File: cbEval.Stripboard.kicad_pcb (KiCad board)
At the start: 2 copper layers, 35 x 109 mm, 33 parts, among them J1 Bergstik-II_3, J10 Socket.Hor.2x5.6-5535512-4, J11 Bergstik-II_3, J12 Bergstik-II_3, J13 Bergstik-II_6, J14 Bergstik-II_8, J15 Bergstik-II_6, J2 Bergstik-II_6, J3 Keystone.4918, J4 Keystone.4918, J5 Keystone.3571, J6 Keystone.3571, J7 Socket.Hor.2x5.6-5535512-4, J8 Header.Hor.2x5.9-103326-0-05, J9 Header.Hor.2x5.9-103326-0-05, U1 SN74AHC138D

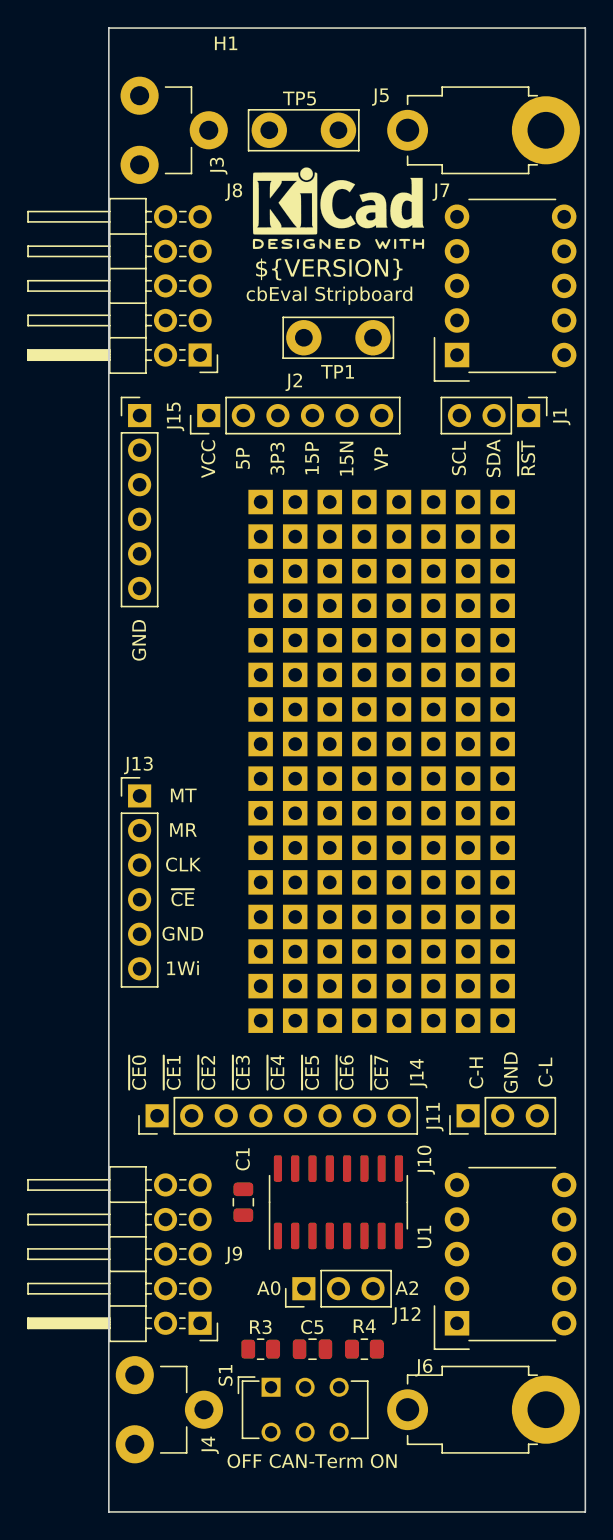
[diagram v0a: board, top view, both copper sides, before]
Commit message: Bus-Stecker getauscht, BOM erstellt
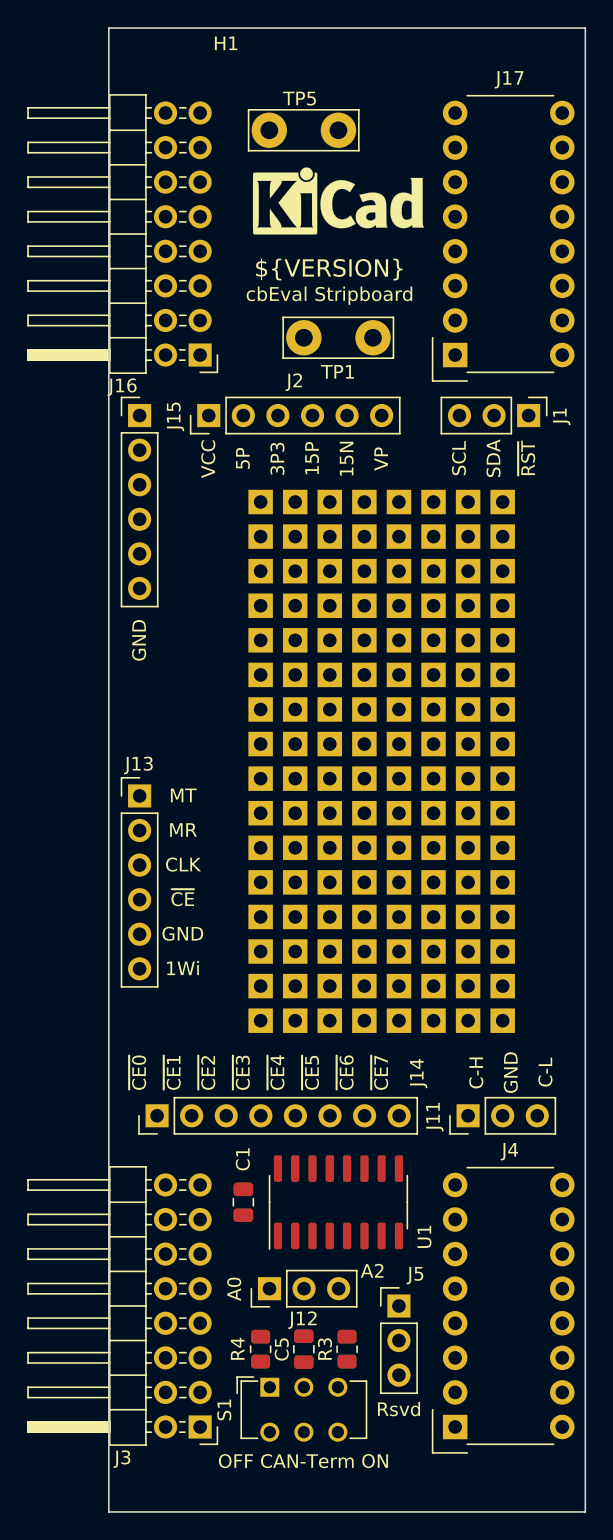
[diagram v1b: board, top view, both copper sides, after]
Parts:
- removed J10, J7: Socket.Hor.2x5.6-5535512-4, BTech.Connector.AMPMODU-ModII:Socket.Hor.2x5.6-5535512-4
- removed J6: Keystone.3571, BTech.Connector.QuickConnect:Keystone.3571
- removed J8, J9: Header.Hor.2x5.9-103326-0-05, Connector_PinHeader_2.54mm:PinHeader_2x05_P2.54mm_Horizontal
- added J16: Header.Hor.2x8.9-103326-0-08, Connector_PinHeader_2.54mm:PinHeader_2x08_P2.54mm_Horizontal, F.Cu at (135.3, 70.5)
- added J17: Socket.Hor.2x8.1-5535512-8, BTech.Connector.AMPMODU-ModII:Socket.Hor.2x5.6-5535512-4, F.Cu at (161.9, 62.9)
- J3: value Keystone.4918 -> Header.Hor.2x8.9-103326-0-08; footprint BTech.Connector.QuickConnect:Keystone.4918 -> Connector_PinHeader_2.54mm:PinHeader_2x08_P2.54mm_Horizontal
- J4: value Keystone.4918 -> Socket.Hor.2x8.1-5535512-8; footprint BTech.Connector.QuickConnect:Keystone.4918 -> BTech.Connector.AMPMODU-ModII:Socket.Hor.2x5.6-5535512-4
- J5: value Keystone.3571 -> Bergstik-II_3; footprint BTech.Connector.QuickConnect:Keystone.3571 -> Connector_PinHeader_2.54mm:PinHeader_1x03_P2.54mm_Vertical
- MP1: footprint Symbol:KiCad-Logo2_5mm_SilkScreen -> Symbol:KiCad-Logo_5mm_SilkScreen
- moved J3 95.4 mm to (135.3, 149.2), turned to 180 degrees
- moved J5 86.5 mm to (149.9, 140.3)
- moved J4 32.0 mm to (161.9, 141.6)
- moved R4 7.62 mm to (139.7, 143.5), turned to 90 degrees
- moved R3 6.35 mm to (146.1, 143.5), turned to -90 degrees
- moved J12 2.53 mm to (140.3, 139.1)
- moved C5 0.63 mm to (142.9, 143.5), turned to -90 degrees
- moved S1 0.09 mm to (140.4, 146.3)
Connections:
- J5 pad 1: GND -> /Reserved0
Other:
- board text added: "Rsvd"

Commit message: Update auf KiCAD-Version 7
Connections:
- net /SPI-~CE renamed /SPI-~{CE}
- net /~RESET renamed /~{RESET}
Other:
- board text added: "~{CE0}"
- board text added: "~{CE1}"
- board text added: "~{CE2}"
- board text added: "~{CE3}"
- board text added: "~{CE4}"
- board text added: "~{CE5}"
- board text added: "~{CE6}"
- board text added: "~{CE7}"
- board text added: "~{CE}"
- board text added: "~{RST}"
- board text removed: "~CE"
- board text removed: "~CE0"
- board text removed: "~CE1"
- board text removed: "~CE2"
- board text removed: "~CE3"
- board text removed: "~CE4"
- board text removed: "~CE5"
- board text removed: "~CE6"
- board text removed: "~CE7"
- board text removed: "~RST"
